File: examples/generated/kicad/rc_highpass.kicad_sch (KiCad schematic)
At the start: 3 parts

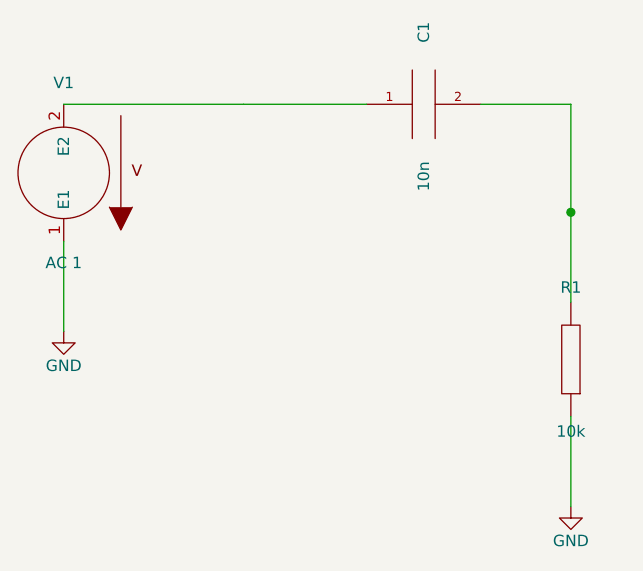
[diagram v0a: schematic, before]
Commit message: Attempt to correct strange wiring.
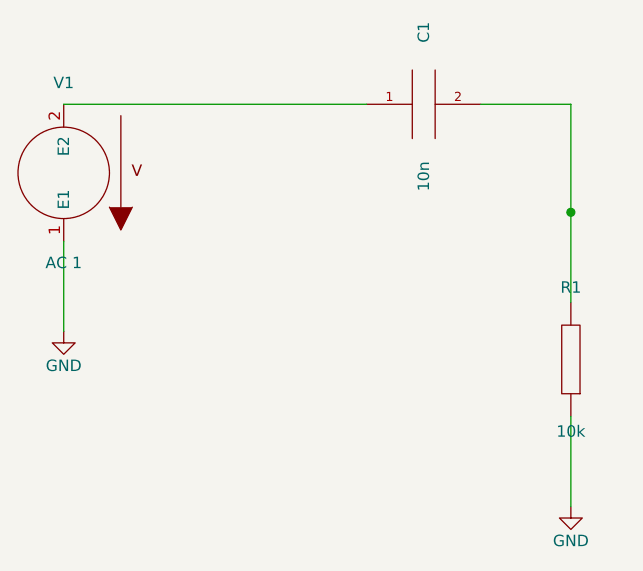
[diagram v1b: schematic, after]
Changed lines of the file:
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@@
     )
   )
-  (wire (pts (xy 50.00 70.38) (xy 70.00 70.38))
+  (wire (pts (xy 50.00 70.38) (xy 83.65 70.38))
     (stroke (width 0) (type solid) (color 0 0 0 0))
   )
-  (wire (pts (xy 83.65 70.38) (xy 70.00 70.38))
-    (stroke (width 0) (type solid) (color 0 0 0 0))
-  )

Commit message: Attempt shape and wiring fixes again.
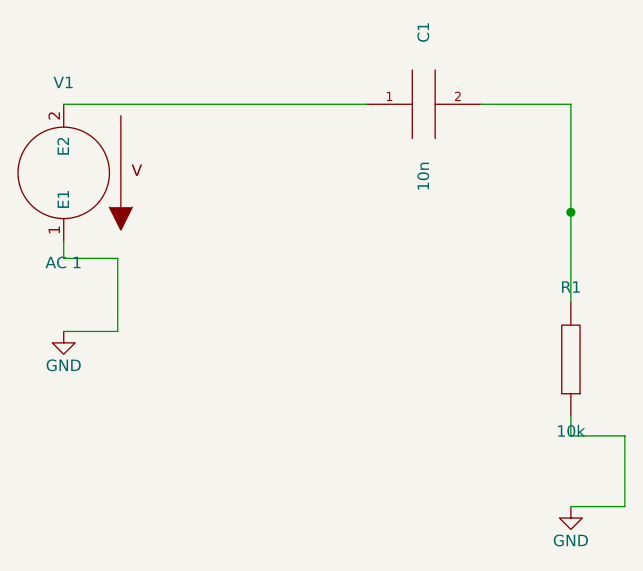
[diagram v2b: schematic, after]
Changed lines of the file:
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@@
     (stroke (width 0) (type solid) (color 0 0 0 0))
   )
-  (wire (pts (xy 50.00 85.62) (xy 50.00 95.62))
+  (wire (pts (xy 50.00 85.62) (xy 50.00 87.50))
     (stroke (width 0) (type solid) (color 0 0 0 0))
   )
-  (wire (pts (xy 106.35 105.08) (xy 106.35 115.08))
+  (wire (pts (xy 50.00 87.50) (xy 56.00 87.50))
     (stroke (width 0) (type solid) (color 0 0 0 0))
   )
+  (wire (pts (xy 56.00 87.50) (xy 56.00 95.62))
+    (stroke (width 0) (type solid) (color 0 0 0 0))
+  )
+  (wire (pts (xy 56.00 95.62) (xy 50.00 95.62))
+    (stroke (width 0) (type solid) (color 0 0 0 0))
+  )
+  (wire (pts (xy 106.35 105.08) (xy 106.35 107.23))
+    (stroke (width 0) (type solid) (color 0 0 0 0))
+  )
+  (wire (pts (xy 106.35 107.23) (xy 112.35 107.23))
+    (stroke (width 0) (type solid) (color 0 0 0 0))
+  )
+  (wire (pts (xy 112.35 107.23) (xy 112.35 115.08))
+    (stroke (width 0) (type solid) (color 0 0 0 0))
+  )
+  (wire (pts (xy 112.35 115.08) (xy 106.35 115.08))
+    (stroke (width 0) (type solid) (color 0 0 0 0))
+  )
